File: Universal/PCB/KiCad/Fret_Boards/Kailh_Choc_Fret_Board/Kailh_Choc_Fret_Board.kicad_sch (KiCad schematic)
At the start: 16 parts, among them SW1 MX_SW_HS, SW2 MX_SW_HS, SW3 MX_SW_HS, SW4 MX_SW_HS, SW5 MX_SW_HS

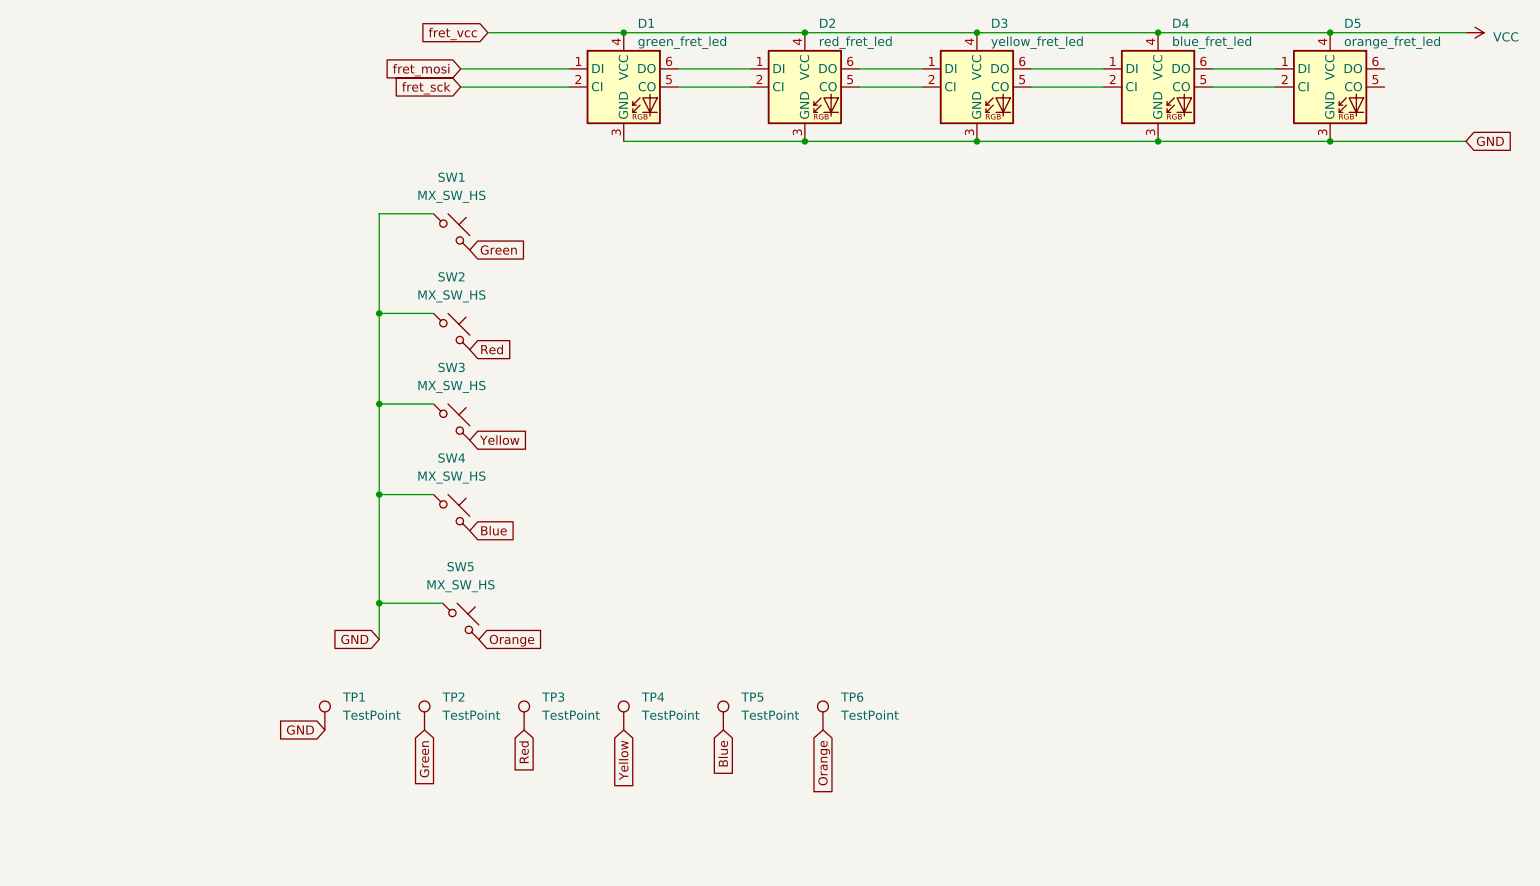
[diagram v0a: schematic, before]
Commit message: updated The choc fret board
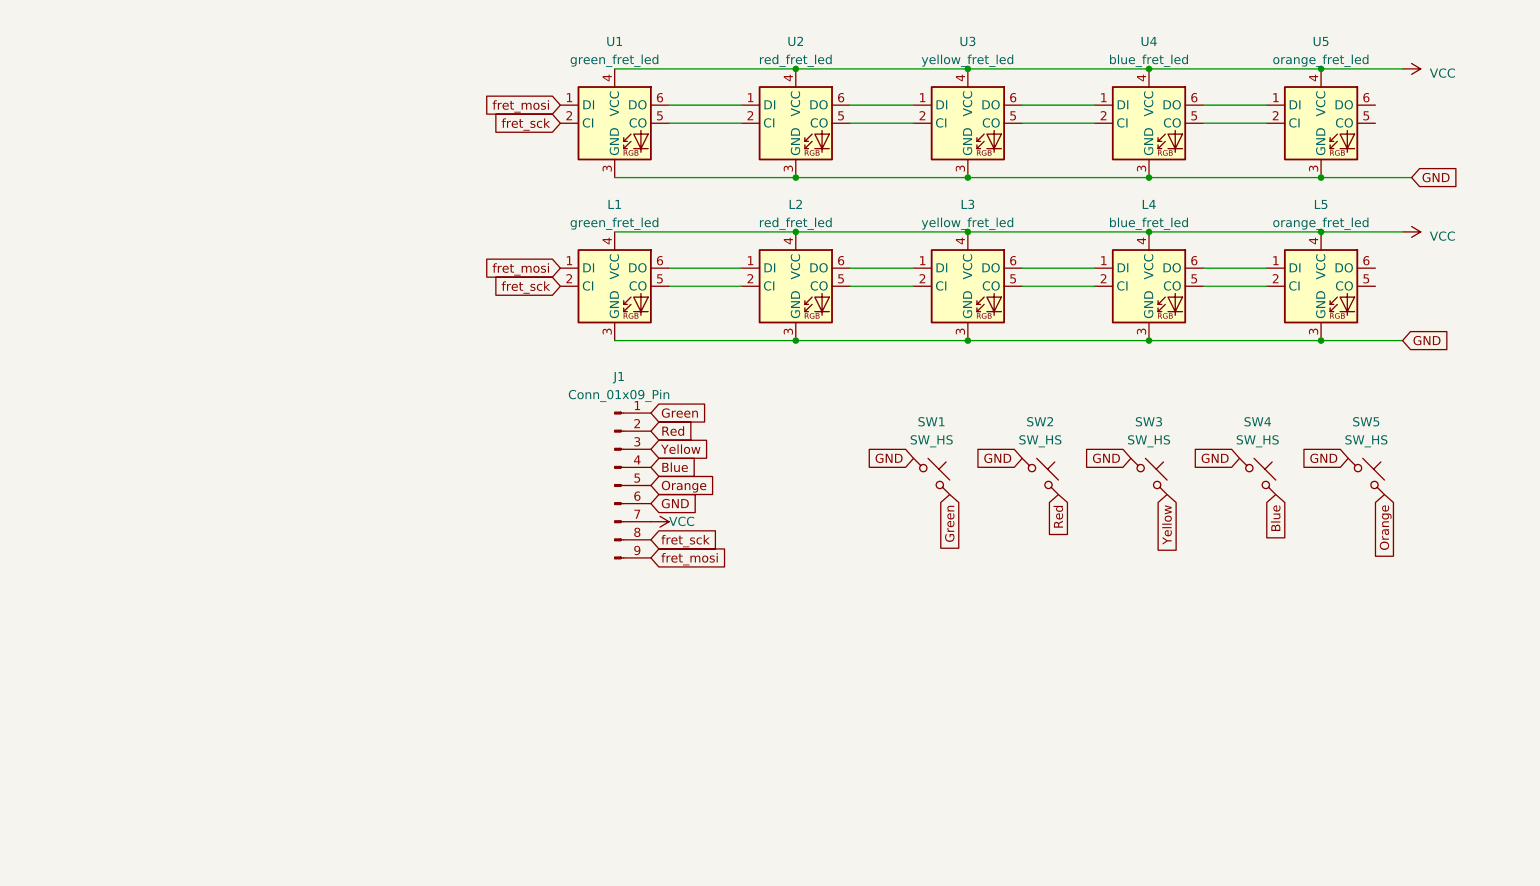
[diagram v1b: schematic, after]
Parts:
- removed TP1, TP2, TP3, TP4, TP5, TP6: TestPoint, symbol Connector:TestPoint
- added J1: Conn_01x09_Pin, Connector_PinHeader_2.54mm:PinHeader_1x09_P2.54mm_Vertical, symbol Connector:Conn_01x09_Pin
- added U1: green_fret_led, LED_SMD:LED_RGB_5050-6, symbol LED:APA102
- added U2: red_fret_led, LED_SMD:LED_RGB_5050-6, symbol LED:APA102
- added U3: yellow_fret_led, LED_SMD:LED_RGB_5050-6, symbol LED:APA102
- added U4: blue_fret_led, LED_SMD:LED_RGB_5050-6, symbol LED:APA102
- added U5: orange_fret_led, LED_SMD:LED_RGB_5050-6, symbol LED:APA102
- SW1, SW2, SW3, SW4, SW5: value MX_SW_HS -> SW_HS; footprint marbastlib-mx:SW_MX_HS_1u -> Minibar:Kailh_Hotswap_Choc
- renumbered D1 to L1, D2 to L2, D3 to L3, D4 to L4, D5 to L5
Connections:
- net Blue: now also J1.4 (Pin_4)
- net GND: now also J1.6 (Pin_6), U1.3 (GND), U2.3 (GND), U3.3 (GND), U4.3 (GND), U5.3 (GND)
- net Green: now also J1.1 (Pin_1)
- net Orange: now also J1.5 (Pin_5)
- net Red: now also J1.2 (Pin_2)
- net VCC: now also J1.7 (Pin_7), U1.4 (VCC), U2.4 (VCC), U3.4 (VCC), U4.4 (VCC), U5.4 (VCC)
- net Yellow: now also J1.3 (Pin_3)
- net fret_mosi: now also J1.9 (Pin_9), U1.1 (DI)
- net fret_sck: now also J1.8 (Pin_8), U1.2 (CI)
- new net: U1.6 (DO), U2.1 (DI)
- new net: U1.5 (CO), U2.2 (CI)
- new net: U2.5 (CO), U3.2 (CI)
- new net: U2.6 (DO), U3.1 (DI)
- new net: U3.5 (CO), U4.2 (CI)
- new net: U3.6 (DO), U4.1 (DI)
- new net: U4.5 (CO), U5.2 (CI)
- new net: U4.6 (DO), U5.1 (DI)
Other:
- moved on the sheet: L1, L2, L3, L4, L5, SW1, SW2, SW3, SW4, SW5

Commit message: updated the MX fret board
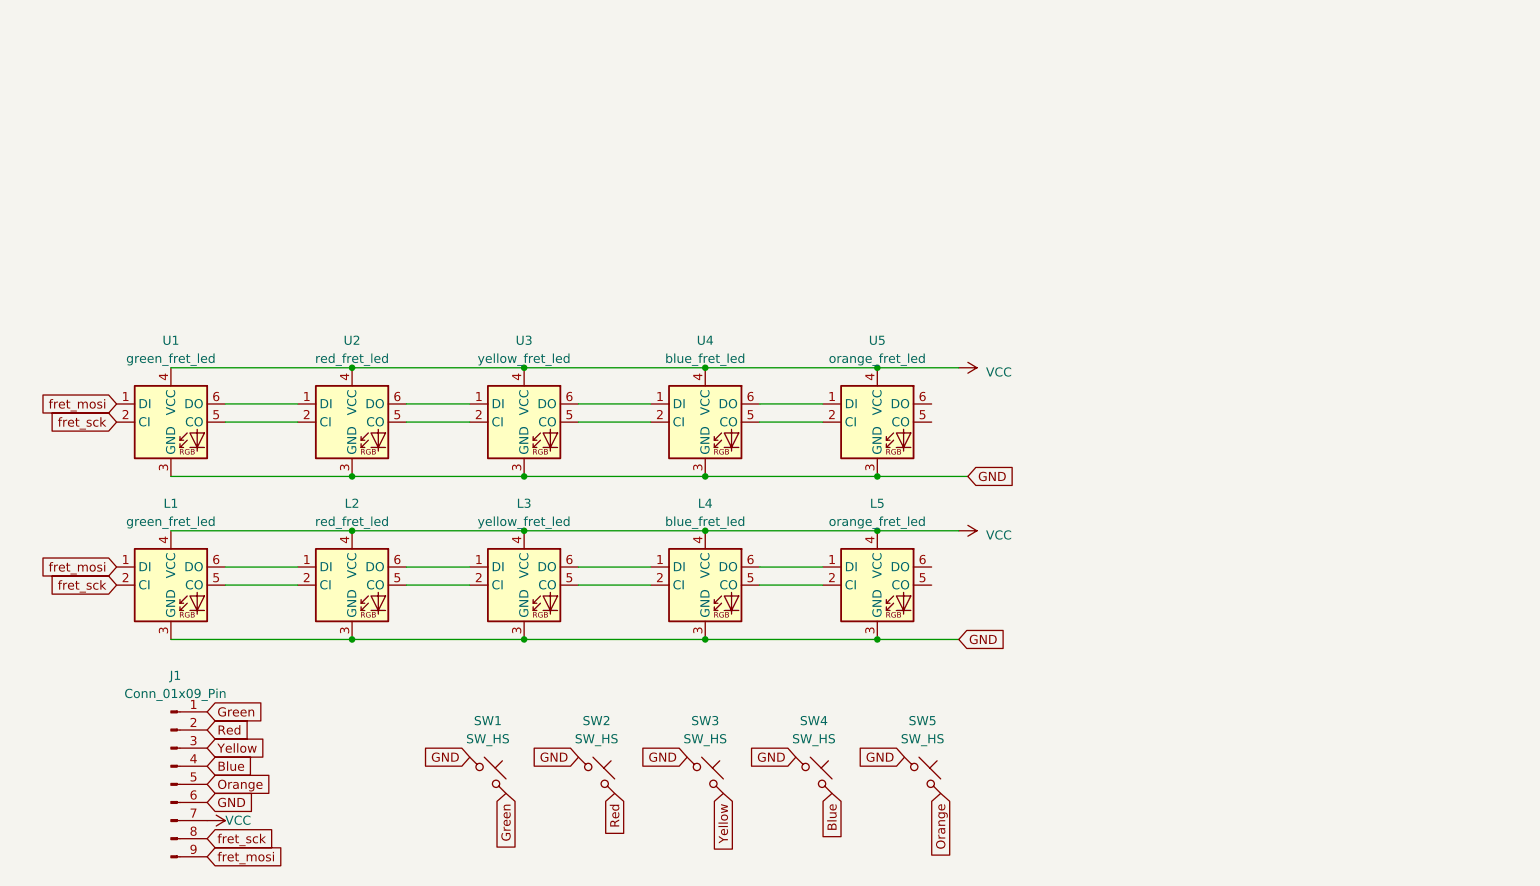
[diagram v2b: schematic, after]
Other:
- moved on the sheet: J1, L1, L2, L3, L4, L5, SW1, SW2, SW3, SW4, SW5, U1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
